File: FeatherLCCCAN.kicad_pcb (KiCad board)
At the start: 2 copper layers, 96.5 x 22.9 mm, 6 parts, among them J301 RJ45, J302 RJ45, U301 TCAN332DR

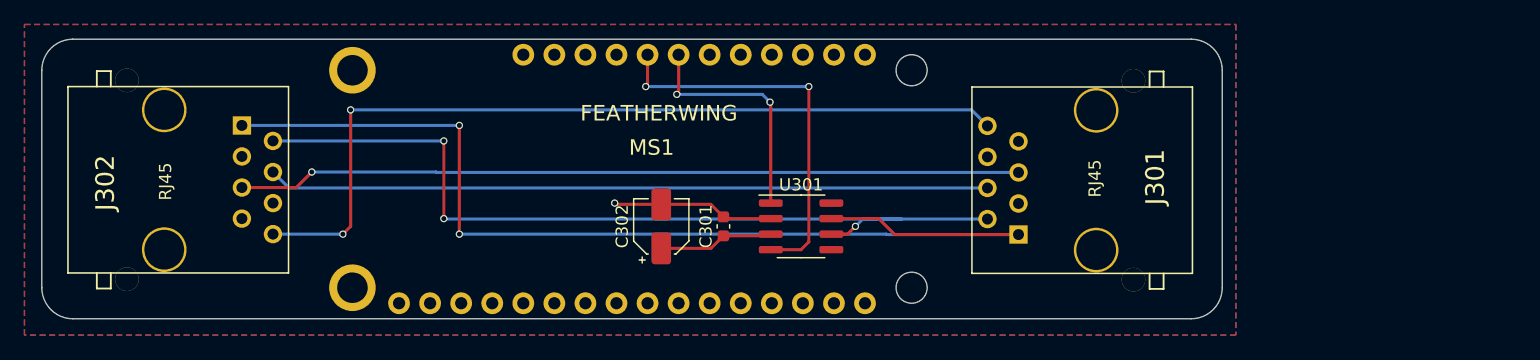
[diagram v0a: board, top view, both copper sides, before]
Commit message: Rev B PCB.
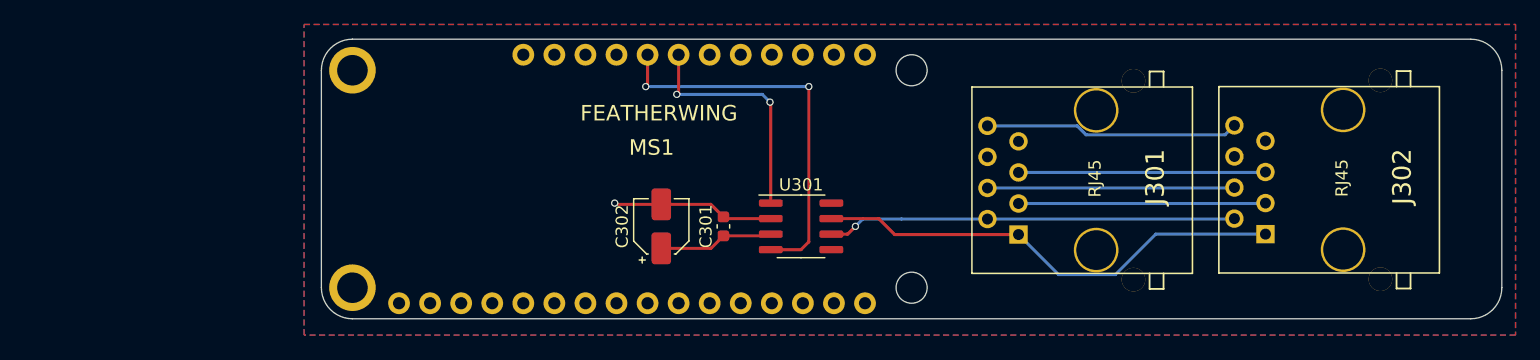
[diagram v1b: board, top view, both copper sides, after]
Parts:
- moved J302 96.4 mm to (206.9, 80.0), turned to 90 degrees
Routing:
- net /CANH: track 88.2 -> 38.8 mm, vias 2 -> 0
- net Net-(J301-Pad8): track 68.7 -> 20.8 mm, vias 2 -> 0
- net Net-(J301-Pad5): track 64.0 -> 20.2 mm, vias 1 -> 0
- net Net-(J301-Pad4): track 59.0 -> 20.2 mm
- net /CANL: track 71.0 -> 33.5 mm, vias 3 -> 1
- net GND: track 13.3 -> 33.5 mm
